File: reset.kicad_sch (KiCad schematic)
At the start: 4 parts, among them SW72 SW_Push, U37 74HC04

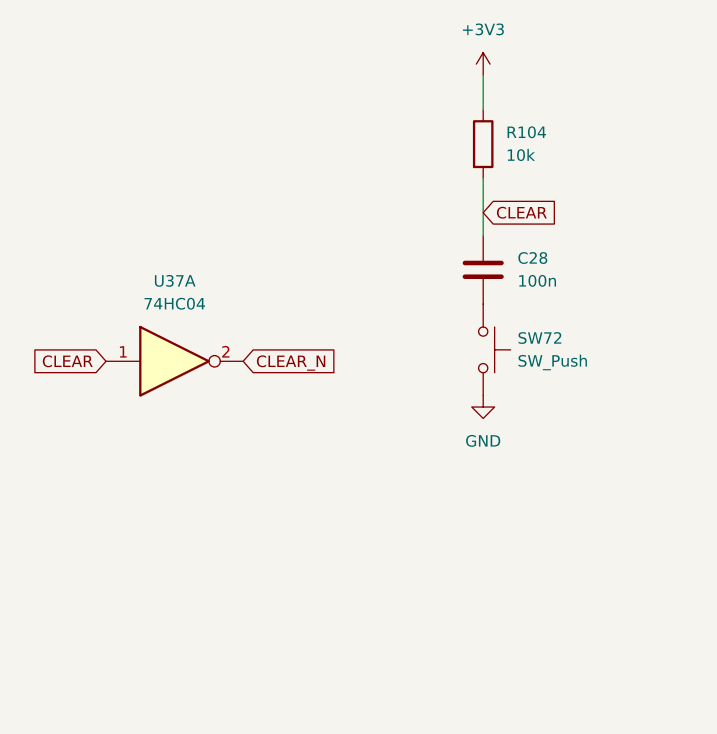
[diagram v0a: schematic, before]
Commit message: very big comit what i did is in the description
jooo so this is what i did i fixed all erc errors now it is basicly finished and also started to make a website where you can lern how this whole thing works and also have a simulation for it but it is still in progress so right now chapter 1 is complete with all the simulations and right now i am working on chapter 6 it should not take very long untill i am finished i will probaply post more comits in the future so yea sry that i forgot to do that ig
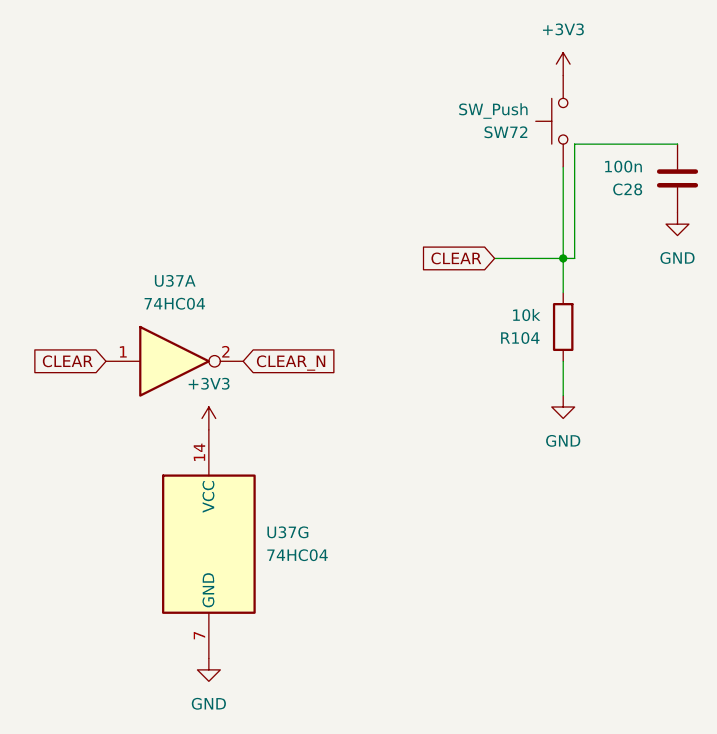
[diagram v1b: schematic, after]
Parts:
- added unit 7 of U37
- U37: footprint Package_DIP:PowerIntegrations_SMD-8C -> (none)
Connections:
- net +3V3: now also SW72.2, U37.14 (VCC); no longer R104.1
- net CLEAR: now also C28.2, SW72.1; no longer C28.1
- net GND: now also C28.1, R104.1, U37.7 (GND); no longer SW72.2
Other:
- moved on the sheet: C28, R104, SW72
